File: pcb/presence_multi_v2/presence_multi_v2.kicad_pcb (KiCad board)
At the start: 2 copper layers, 32 parts, among them IC1 LDL1117S33R, J1 USB_C_Receptacle_USB2.0_16P, J2 TC2050, J3 Conn_01x06_Socket, U3 CH340E, Y1 Wurth 830050789

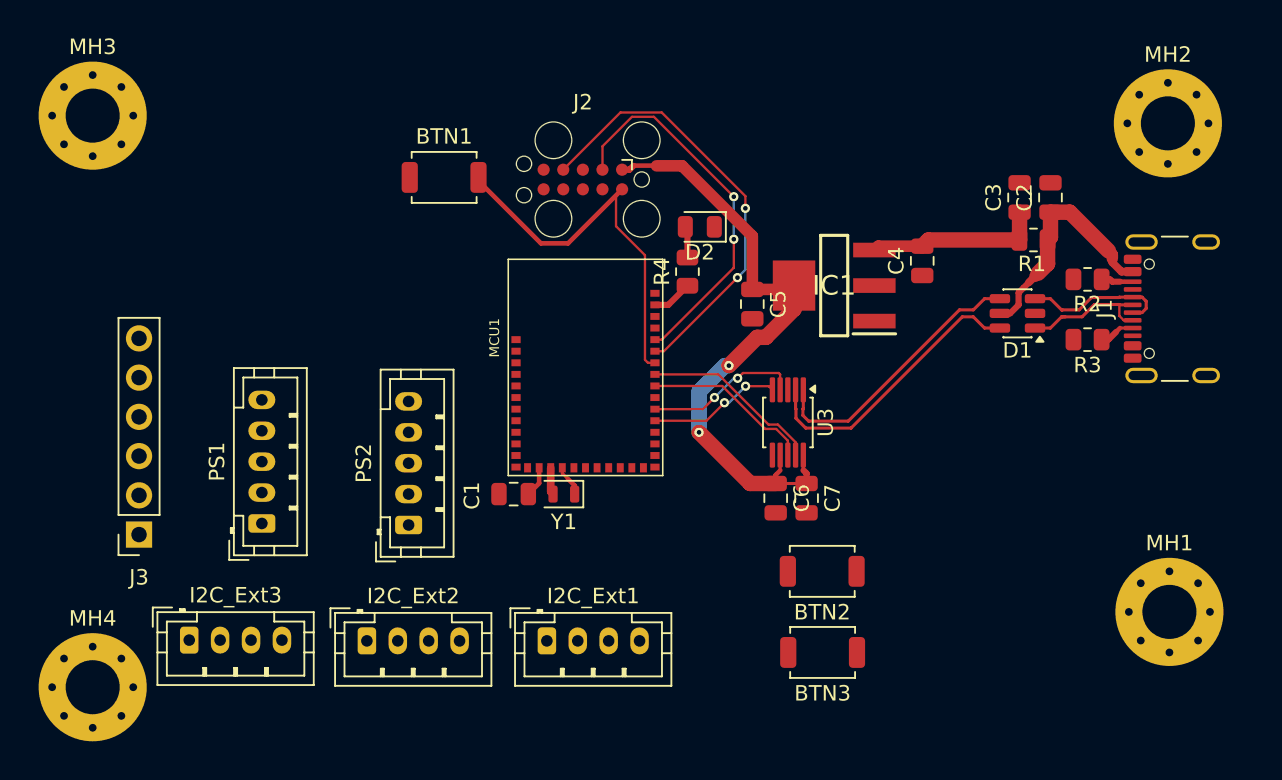
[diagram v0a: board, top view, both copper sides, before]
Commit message: ready version
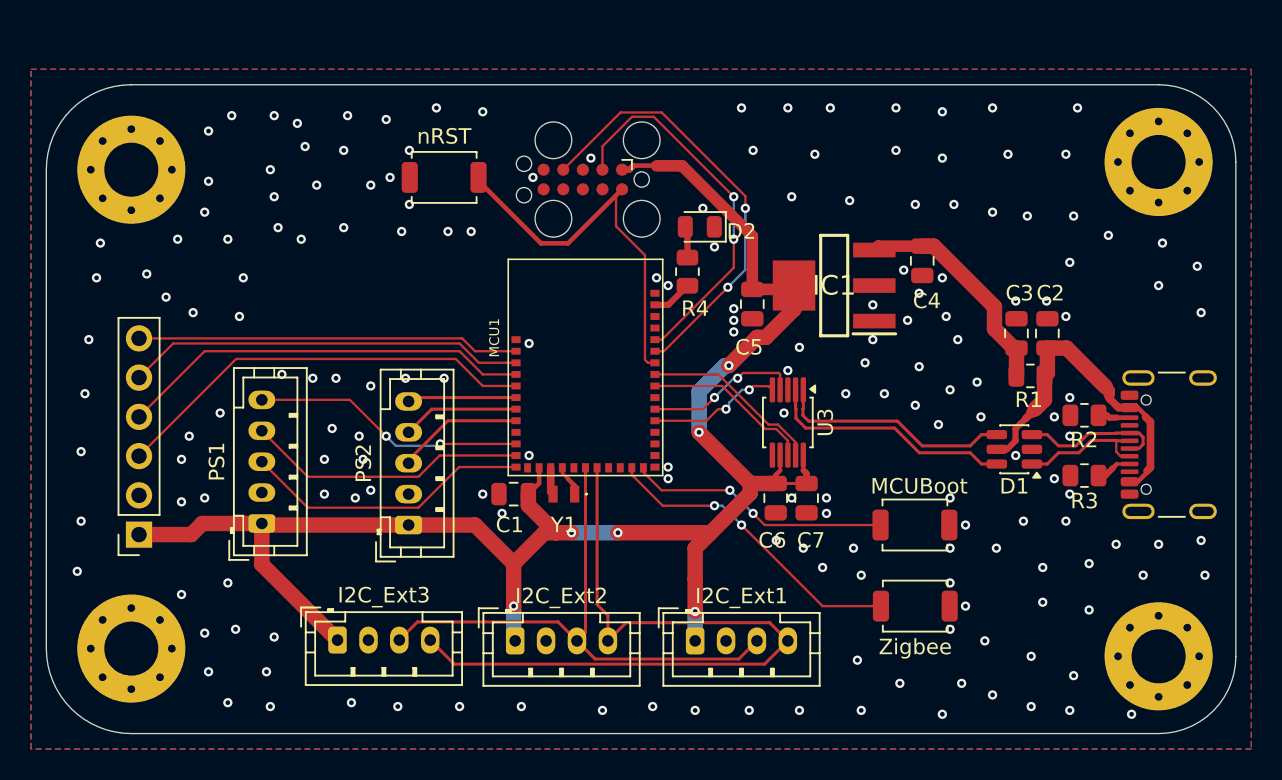
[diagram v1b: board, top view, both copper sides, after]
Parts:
- Y1: footprint Crystal:Crystal_SMD_2012-2Pin_2.0x1.2mm -> theorlangur:Wurth-XTAL-830050789
- moved I2C_Ext1 9.60 mm to (129.0, 123.0)
- moved I2C_Ext2 9.60 mm to (117.3, 123.0)
- moved I2C_Ext3 9.60 mm to (105.8, 123.0)
- moved R2 8.80 mm to (154.2, 108.4)
- moved D1 8.80 mm to (149.7, 110.6)
- moved R1 8.80 mm to (150.7, 105.8)
- moved R3 8.80 mm to (154.2, 112.3)
- moved C2 8.80 mm to (151.8, 103.1)
- moved C3 8.80 mm to (149.8, 103.1)
- moved J1 8.80 mm to (160.8, 110.3)
- moved MCUBoot 6.71 mm to (143.2, 115.5)
- moved Zigbee 6.71 mm to (143.2, 120.8)
- moved MH3 4.30 mm to (92.5, 92.5)
- moved MH4 3.54 mm to (92.5, 123.5)
- moved MH1 2.96 mm to (159.0, 124.0)
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- renumbered BTN2 to MCUBoot, BTN3 to Zigbee, BTN1 to nRST
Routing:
- net +3V3: track 43.7 -> 112.5 mm, vias 2 -> 6
- net /I2C20_SDA: track 0.00 -> 48.5 mm
- net /I2C20_SCL: track 0.00 -> 36.5 mm
- net /EXT0: track 0.00 -> 27.7 mm
- net /EXT1: track 0.00 -> 26.8 mm
- net /EXT2: track 0.00 -> 25.8 mm
- net /EXT3: track 0.00 -> 24.7 mm
- net /BTN_ZB: track 0.00 -> 20.1 mm, vias 0 -> 2
- net /UART20_TX: track 0.00 -> 18.8 mm
- net /UART20_RX: track 0.00 -> 18.3 mm
- net /I_PRESENCE1: track 0.00 -> 17.7 mm, vias 0 -> 2
- net /BTN_MCUBoot: track 0.00 -> 17.1 mm, vias 0 -> 2
- net /UART21_TX: track 0.00 -> 8.21 mm
- net /UART21_RX: track 0.00 -> 7.57 mm
- net /I_PRESENCE2: track 0.00 -> 7.06 mm
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- added copper zone on B.Cu, net GND
- added copper zone on F.Cu, net GND
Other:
- board outline added: 77 x 42 mm
